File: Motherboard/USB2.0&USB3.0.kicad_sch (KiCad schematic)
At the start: 11 parts, among them J4 USB3_A_Stacked, U3 ULC0524P, U5 ULC0524P

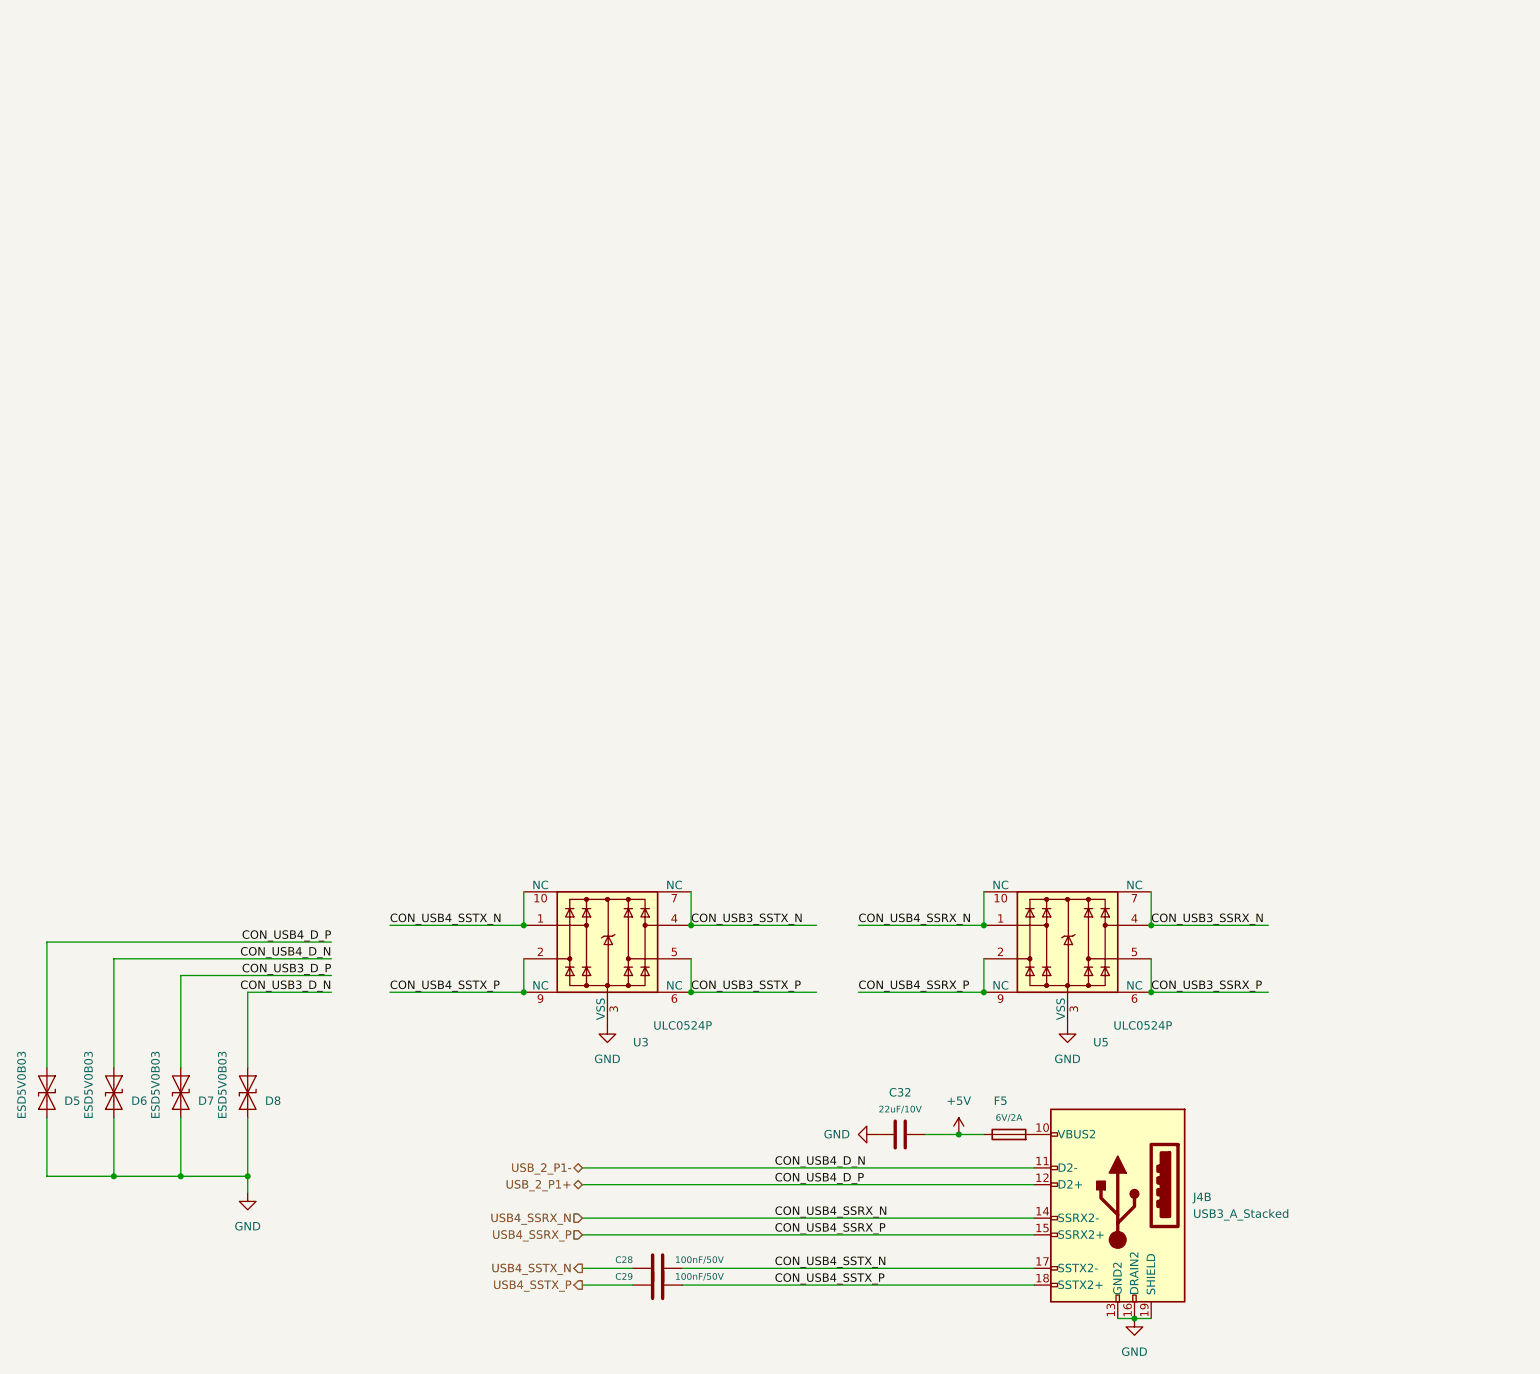
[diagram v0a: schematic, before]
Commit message: Motherboard Complete (aside from parts-BOM associations)
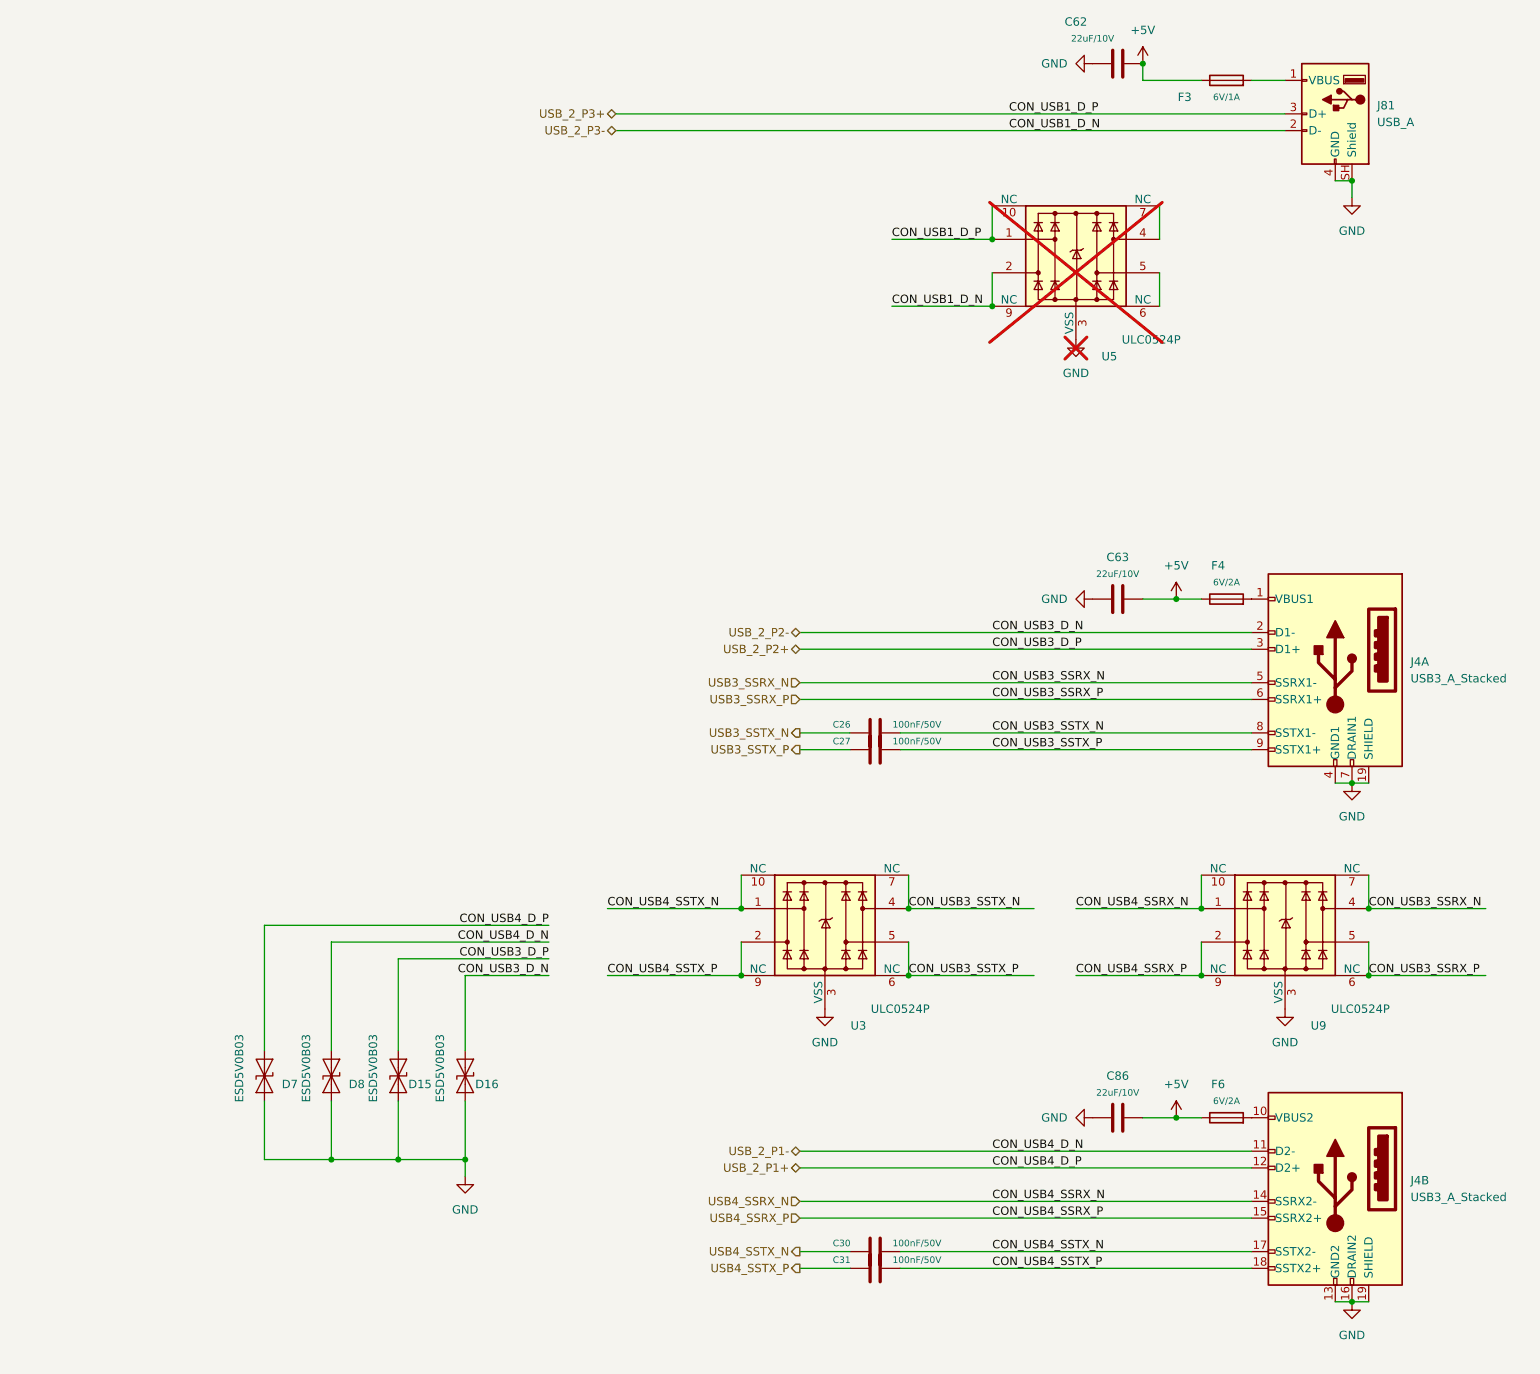
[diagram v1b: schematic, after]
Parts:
- removed C28, C29: 100nF/50V, A_HDJ_Library:C_0402_1005Metric, symbol Device:C
- removed C32: 22uF/10V, A_HDJ_Library:C_0603_1608Metric, symbol Device:C
- removed D5, D6: ESD5V0B03, A_HDJ_Library:D_0402_1005Metric, symbol Diode:ESD9B5.0ST5G
- removed F5: 6V/2A, A_HDJ_Library:Fuse_0805_2012Metric, symbol Device:Fuse
- added C26, C27, C30, C31: 100nF/50V, A_HDJ_Library:C_0402_1005Metric, symbol Device:C
- added C62, C63, C86: 22uF/10V, A_HDJ_Library:C_0603_1608Metric, symbol Device:C
- added D15, D16: ESD5V0B03, A_HDJ_Library:D_0402_1005Metric, symbol Diode:ESD9B5.0ST5G
- added F3: 6V/1A, A_HDJ_Library:Fuse_0805_2012Metric, symbol Device:Fuse
- added F4: 6V/2A, A_HDJ_Library:R_0805_2012Metric, symbol Device:Fuse
- added F6: 6V/2A, A_HDJ_Library:Fuse_0805_2012Metric, symbol Device:Fuse
- added unit 1 of J4
- added J81: USB_A, symbol Connector:USB_A
- added U9: ULC0524P, A_HDJ_Library:Diodes_UDFN-10_1.0x2.5mm_P0.5mm, symbol Power_Protection:D3V3XA4B10LP
- U5: now not fitted; now left out of the parts list
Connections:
- net CON_USB3_D_N is gone; now on net USB_2_P1-: D8.2 (A2)
- net CON_USB3_D_P is gone; now on net USB_2_P1+: D7.2 (A2)
- net +5V: now also C62.2, C63.2, C86.2, F3.1, F4.1, F6.1
- net CON_USB3_SSTX_N: now also C26.2, J4.8 (SSTX1-)
- net CON_USB3_SSTX_P: now also C27.2, J4.9 (SSTX1+)
- net CON_USB4_SSTX_N: now also C30.2
- net CON_USB4_SSTX_P: now also C31.2
- net GND: now also C62.1, C63.1, C86.1, D15.1 (A1), D16.1 (A1), J4.19 (SHIELD), J4.4 (GND1), J4.7 (DRAIN1), J81.4 (GND), J81.SH (Shield), U9.3 (VSS), U9.8 (VSS)
- net USB4_SSRX_N: now also U9.1, U9.10 (NC); no longer U5.1, U5.10 (NC)
- net USB4_SSRX_P: now also U9.2, U9.9 (NC); no longer U5.2, U5.9 (NC)
- net USB4_SSTX_N: now also C30.1
- net USB4_SSTX_P: now also C31.1
- net at J4.10 (VBUS2): now also F6.2
- net CON_USB3_SSRX_N: no longer names the net of U5.4, U5.7 (NC)
- net CON_USB3_SSRX_P: no longer names the net of U5.5, U5.6 (NC)
- new net: F4.2, J4.1 (VBUS1)
- new net: F3.2, J81.1 (VBUS)
- new net USB3_SSRX_N: J4.5 (SSRX1-), U9.4, U9.7 (NC)
- new net USB3_SSRX_P: J4.6 (SSRX1+), U9.5, U9.6 (NC)
- new net USB3_SSTX_N: C26.1
- new net USB3_SSTX_P: C27.1
- new net USB_2_P2+: D15.2 (A2), J4.3 (D1+)
- new net USB_2_P2-: D16.2 (A2), J4.2 (D1-)
- new net USB_2_P3+: J81.3 (D+), U5.1, U5.10 (NC)
- new net USB_2_P3-: J81.2 (D-), U5.2, U5.9 (NC)
